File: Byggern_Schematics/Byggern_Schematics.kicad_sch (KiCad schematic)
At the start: 17 parts, among them J3 V_{In} Plug, J4 GND Plug, J6 IO_Board, SW1 Reset, U1 ATmega162-16P, U2 LM7805_TO220, Y1 4.9152MHz

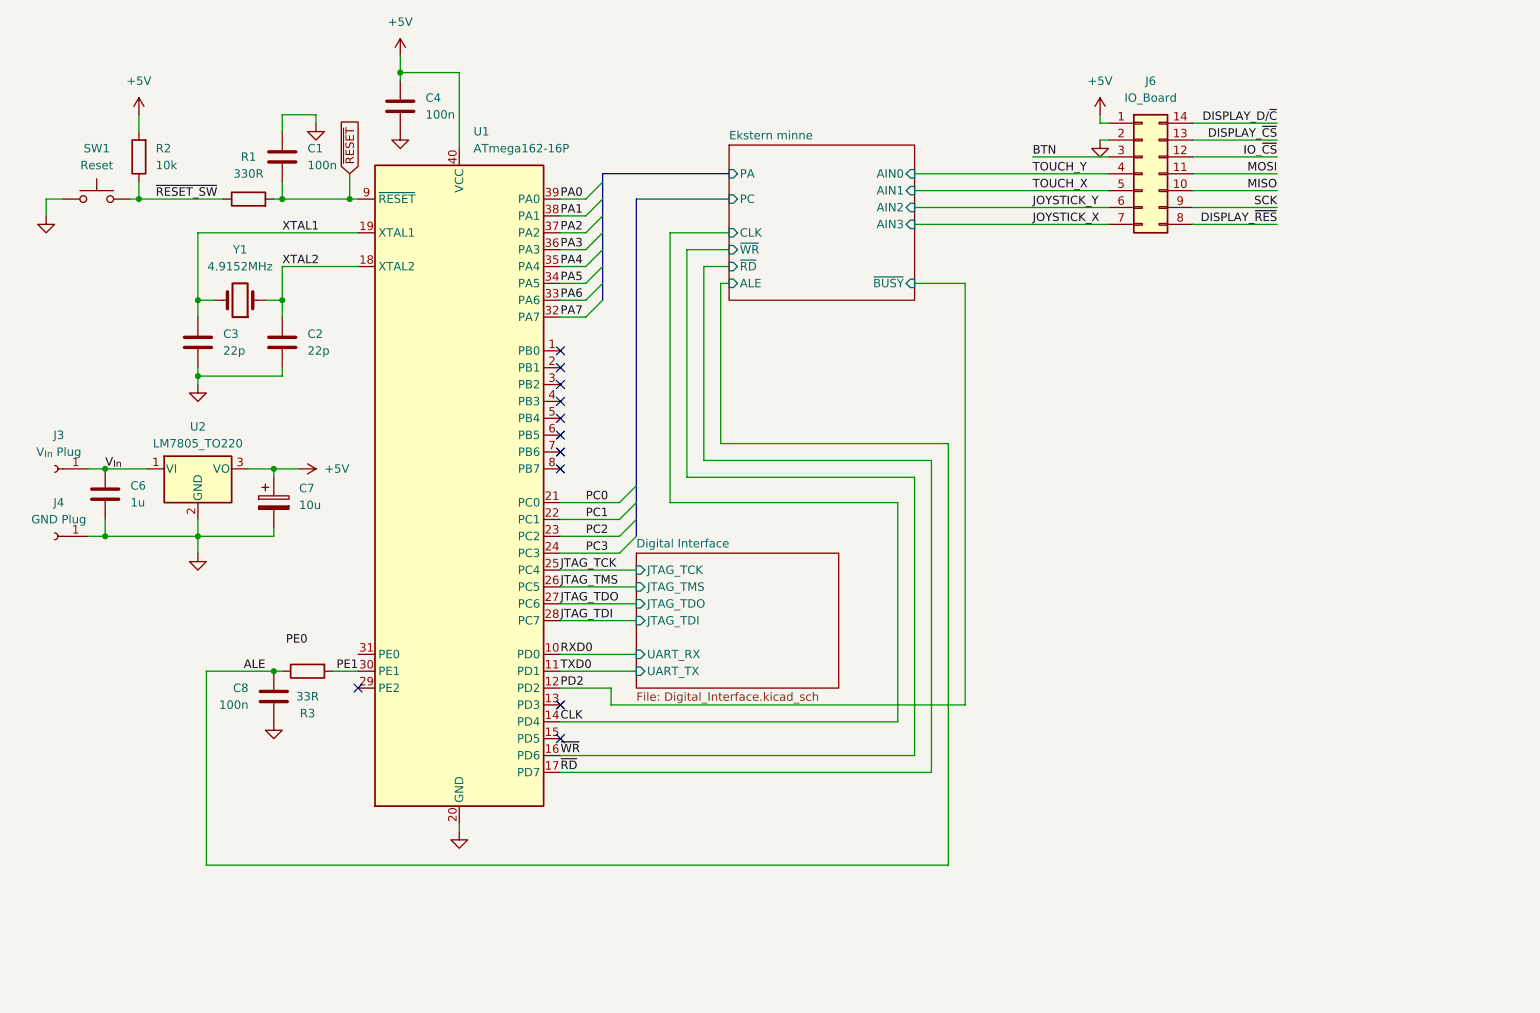
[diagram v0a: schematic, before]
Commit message: Schematic udated
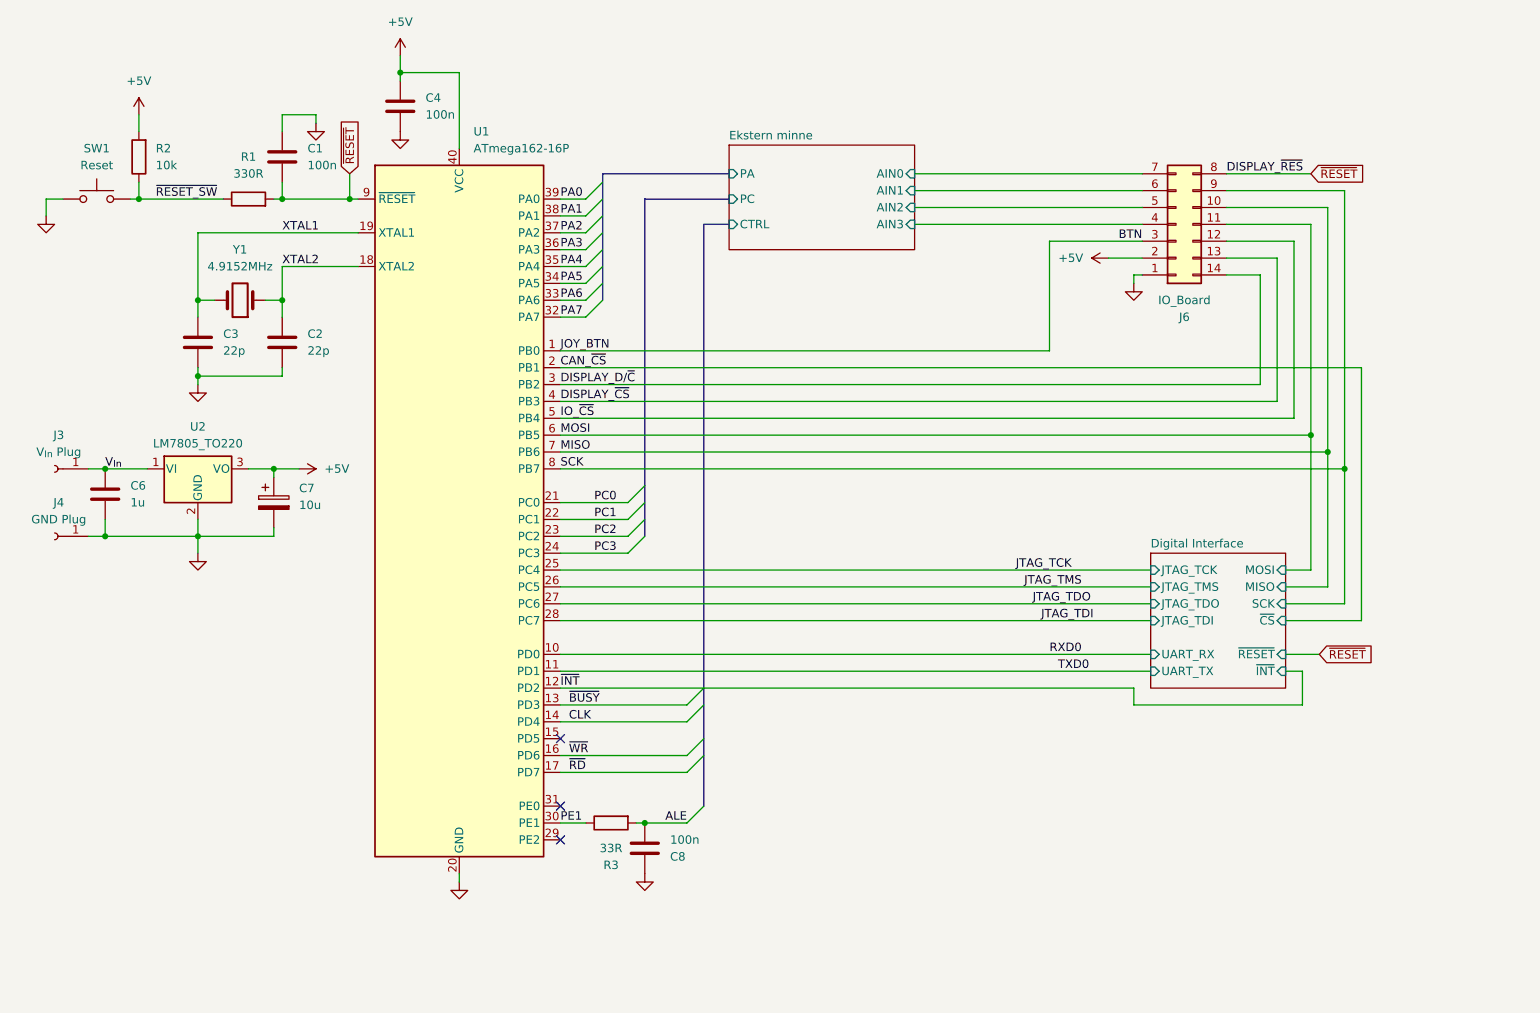
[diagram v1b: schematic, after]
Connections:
- net DISPLAY_~{RES} is gone; now on net ~{RESET}: J6.8 (Pin_8)
- net +5V: now also J6.2 (Pin_2); no longer J6.1 (Pin_1)
- net ALE: now also C8.1, R3.2; no longer C8.2, R3.1
- net BTN: now also U1.1 (PB0)
- net DISPLAY_D/~{C}: now also U1.3 (PB2)
- net DISPLAY_~{CS}: now also U1.4 (PB3)
- net GND: now also C8.2, J6.1 (Pin_1); no longer C8.1, J6.2 (Pin_2)
- net IO_~{CS}: now also U1.5 (PB4)
- net MISO: now also U1.7 (PB6)
- net MOSI: now also U1.6 (PB5)
- net PE1: now also R3.1; no longer R3.2
- net SCK: now also U1.8 (PB7)
- net ~{BUSY}: now reaches U1.13 (PD3)
- net CAN_~{CS}: now reaches U1.2 (PB1)
- net JOYSTICK_X renamed Ekstern minne/AIN0
- net JOYSTICK_Y renamed Ekstern minne/AIN1
- net PD2 renamed ~{INT}
- net TOUCH_X renamed Ekstern minne/AIN2
- net TOUCH_Y renamed Ekstern minne/AIN3
- no-connect marks 11 -> 3
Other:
- sheet Digital Interface ports: added MISO, MOSI, SCK, ~{CS}, ~{INT}, ~{RESET}; removed none
- sheet Ekstern minne ports: added CTRL; removed ALE, CLK, ~{BUSY}, ~{RD}, ~{WR}
- moved on the sheet: U1

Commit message: Finnished schematic
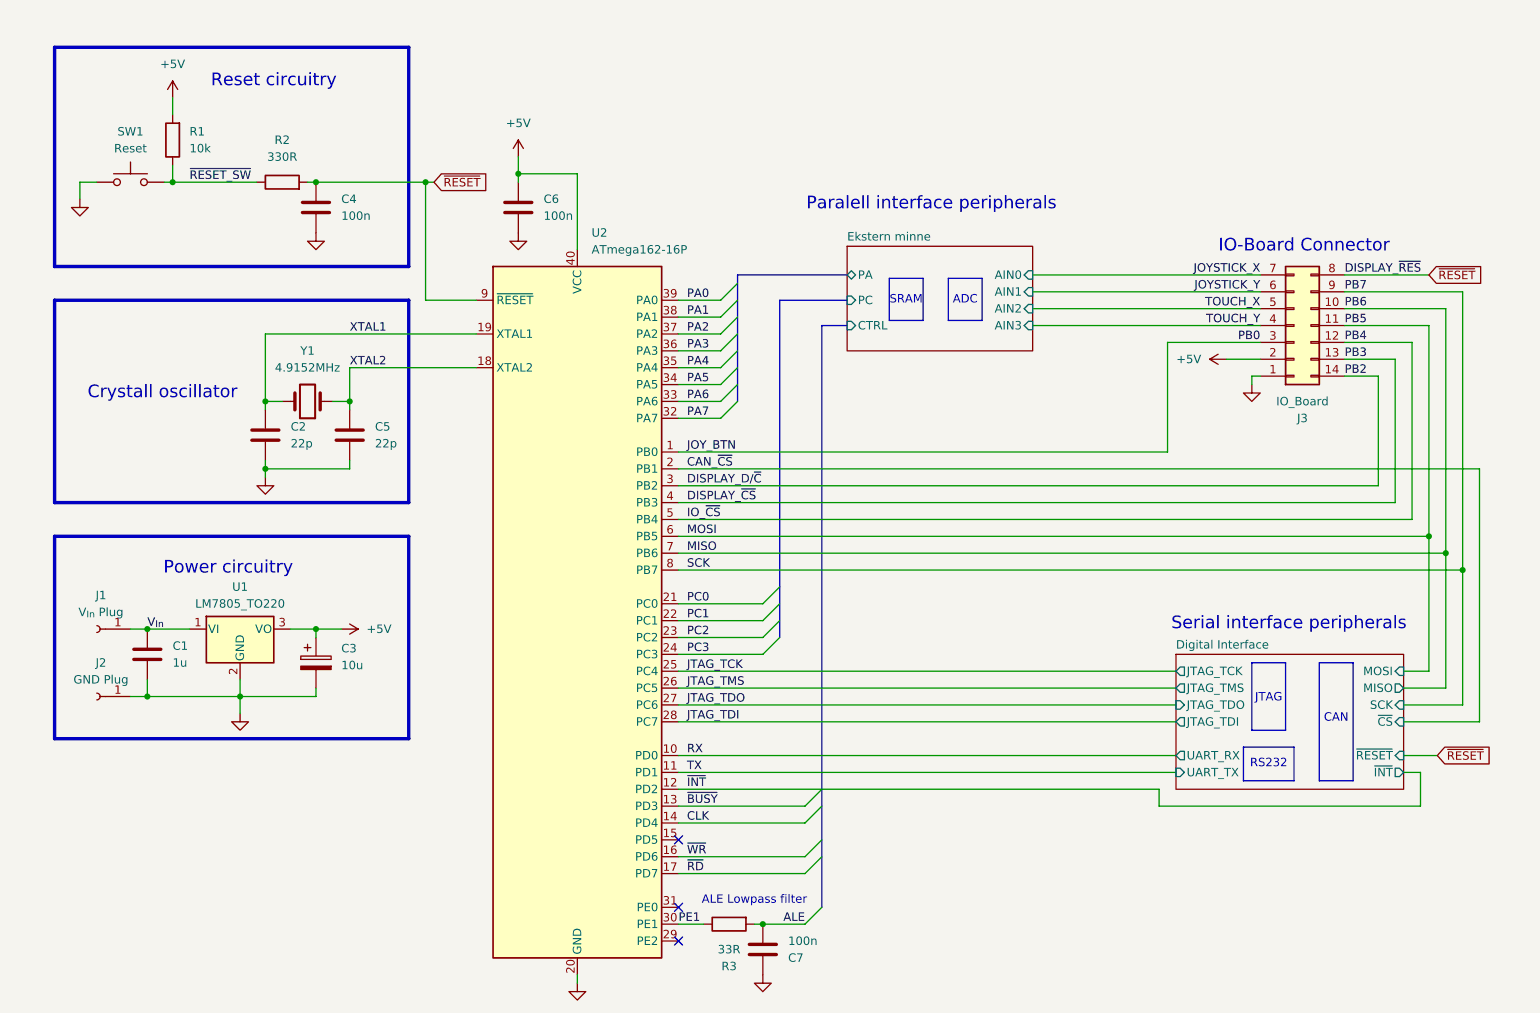
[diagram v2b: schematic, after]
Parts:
- removed C1: 100n, symbol Device:C
- added C4: 100n, symbol Device:C
- renumbered C6 to C1, C3 to C2, C7 to C3, C2 to C5, C4 to C6, C8 to C7, J3 to J1, J4 to J2, J6 to J3, R2 to R1, R1 to R2, U2 to U1, U1 to U2
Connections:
- net GND: now also C4.2
- net ~{RESET}: now also C4.1
- net BTN renamed JOY_BTN
- net Ekstern minne/AIN0 renamed JOYSTICK_X
- net Ekstern minne/AIN1 renamed JOYSTICK_Y
- net Ekstern minne/AIN2 renamed TOUCH_X
- net Ekstern minne/AIN3 renamed TOUCH_Y
- net RXD0 renamed RX
- net SCK renamed PB7
- net TXD0 renamed TX
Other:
- note added: "ADC"
- note added: "ALE Lowpass filter"
- note added: "CAN"
- note added: "Crystall oscillator"
- note added: "IO-Board Connector"
- note added: "JTAG"
- note added: "Paralell interface peripherals"
- note added: "Power circuitry"
- note added: "RS232"
- note added: "Reset circuitry"
- note added: "SRAM"
- note added: "Serial interface peripherals"
- company: (none) -> Gruppe 31
- title: Peneste shittet ever -> Veldig pent yup yup
- moved on the sheet: C1, C2, C3, C5, C6, C7, J1, J2, J3, R1, R2, R3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
